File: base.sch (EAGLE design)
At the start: 20 parts

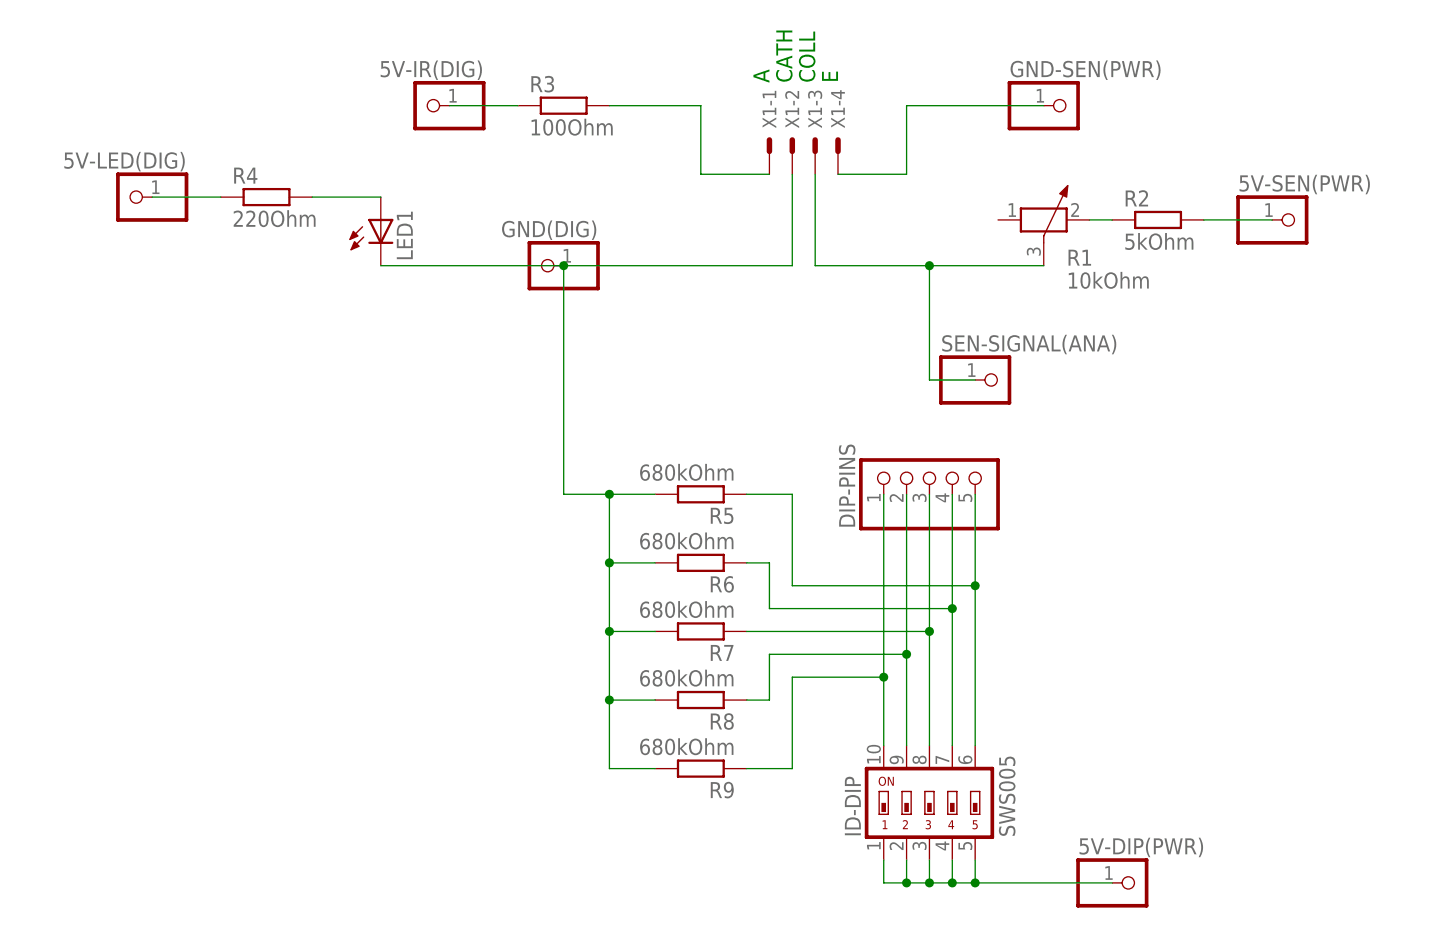
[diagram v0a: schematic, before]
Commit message: no message
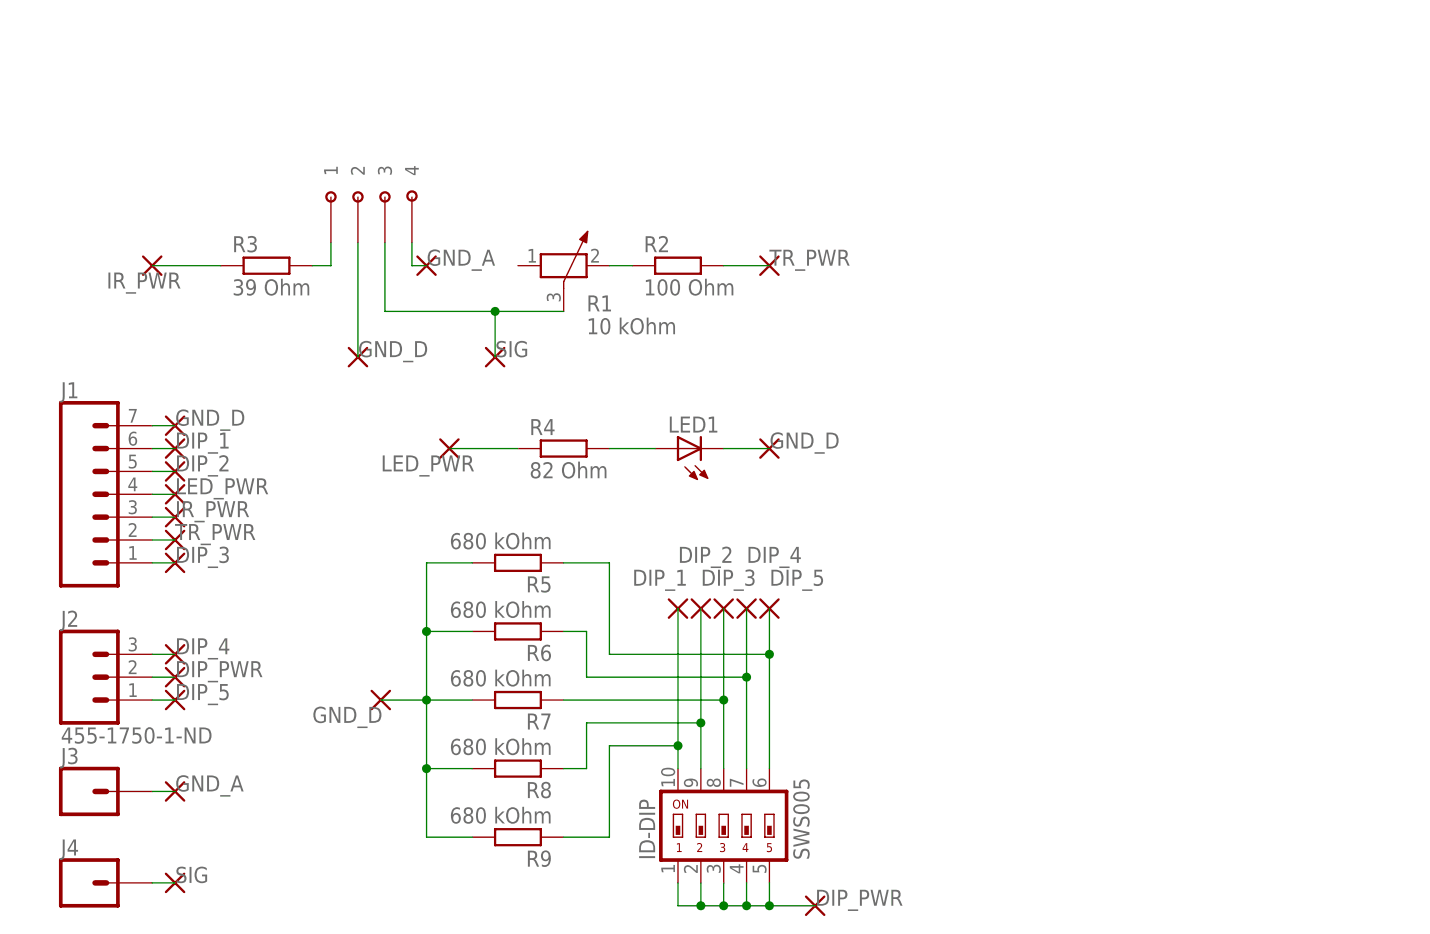
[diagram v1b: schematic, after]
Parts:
- removed 5V-DIP(PWR), 5V-IR(DIG), 5V-LED(DIG), 5V-SEN(PWR), GND(DIG), GND-SEN(PWR), SEN-SIGNAL(ANA): (no value), pinhead:PINHD-1X1
- removed DIP-PINS: (no value), pinhead:PINHD-1X5
- removed X1: (no value), con-molex:KK-156-4
- added J1: (no value), SparkFun-Connectors:CONN_07
- added J2: 455-1750-1-ND, SparkFun-Connectors:CONN_03
- added J3, J4: (no value), SparkFun-Connectors:CONN_01
- added U$4: DF1BZ-4DP-2.5DSA, ferraris_sensor_project:DF1BZ-4DP-2.5DSA
- R1: value 10kOhm -> 10 kOhm
- R2: value 5kOhm -> 100 Ohm
- R3: value 100Ohm -> 39 Ohm
- R4: value 220Ohm -> 82 Ohm
- R5, R6, R7, R8, R9: value 680kOhm -> 680 kOhm
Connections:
- removed net N$10: 5V-DIP(PWR).1, ID-DIP.1, ID-DIP.2, ID-DIP.3, ID-DIP.4, ID-DIP.5
- removed net N$11: DIP-PINS.1, ID-DIP.10, R9.1
- removed net N$12: DIP-PINS.2, ID-DIP.9, R8.1
- removed net N$13: DIP-PINS.3, ID-DIP.8, R7.1
- removed net N$14: DIP-PINS.4, ID-DIP.7, R6.1
- removed net N$15: DIP-PINS.5, ID-DIP.6, R5.1
- removed net N$16: GND(DIG).1, LED1.C, R5.2, R6.2, R7.2, R8.2, R9.2, X1-2.S
- removed net N$4: R3.2, X1-1.S
- removed net N$5: 5V-IR(DIG).1, R3.1
- removed net N$6: 5V-LED(DIG).1, R4.1
- removed net N$8: GND-SEN(PWR).1, X1-4.S
- removed net N$9: 5V-SEN(PWR).1, R2.2
- new net DIP_1: ID-DIP.10, J1.6, R9.1
- new net DIP_2: ID-DIP.9, J1.5, R8.1
- new net DIP_3: ID-DIP.8, J1.1, R7.1
- new net DIP_4: ID-DIP.7, J2.3, R6.1
- new net DIP_5: ID-DIP.6, J2.1, R5.1
- new net DIP_PWR: ID-DIP.1, ID-DIP.2, ID-DIP.3, ID-DIP.4, ID-DIP.5, J2.2
- new net GND_A: J3.1, U$4.4
- new net GND_D: J1.7, LED1.C, R5.2, R6.2, R7.2, R8.2, R9.2, U$4.2
- new net IR_PWR: J1.3, R3.1
- new net LED_PWR: J1.4, R4.1
- new net SIG: J4.1, R1.3, U$4.3
- new net TR_PWR: J1.2, R2.2
- net N$2: now also R3.2, U$4.1; no longer R1.3, SEN-SIGNAL(ANA).1, X1-3.S
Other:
- note removed: "A"
- note removed: "CATH"
- note removed: "COLL"
- note removed: "E"
- moved on the sheet: ID-DIP, LED1, R1, R2, R3, R4, R5, R6, R7, R8, R9
